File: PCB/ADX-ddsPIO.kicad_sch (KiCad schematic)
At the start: 71 parts, among them J1 Conn_Coaxial, J2 +12V, Q1 BS170, Q2 BS170, Q3 BS170, Q5 BS170, U1 L7805, U2 74LS244, U4 CD2003GB_GP

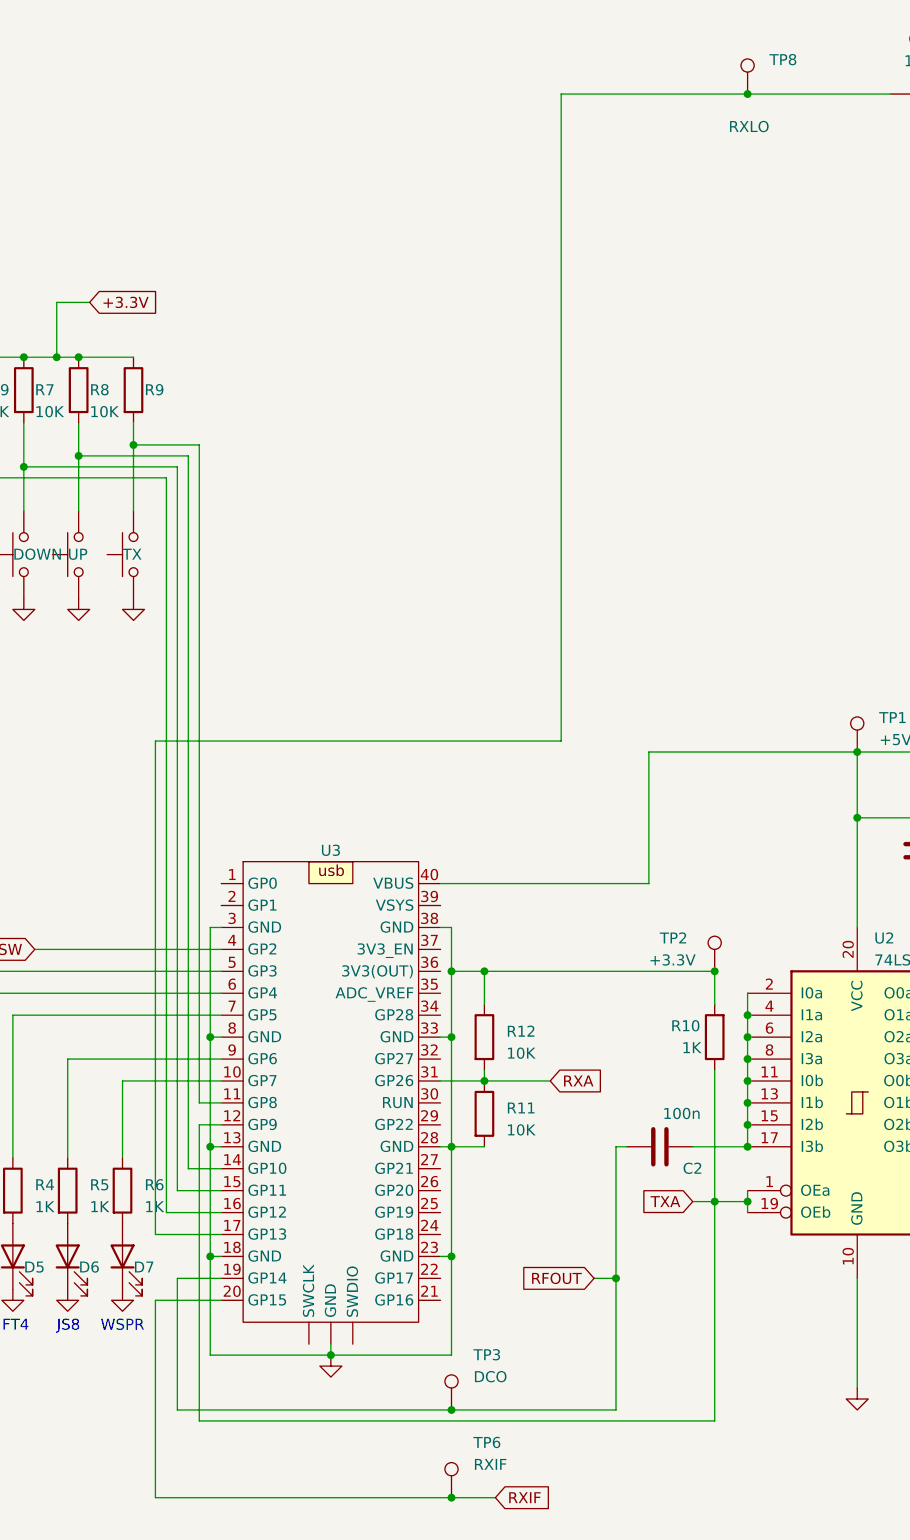
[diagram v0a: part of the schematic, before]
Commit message: dualclk
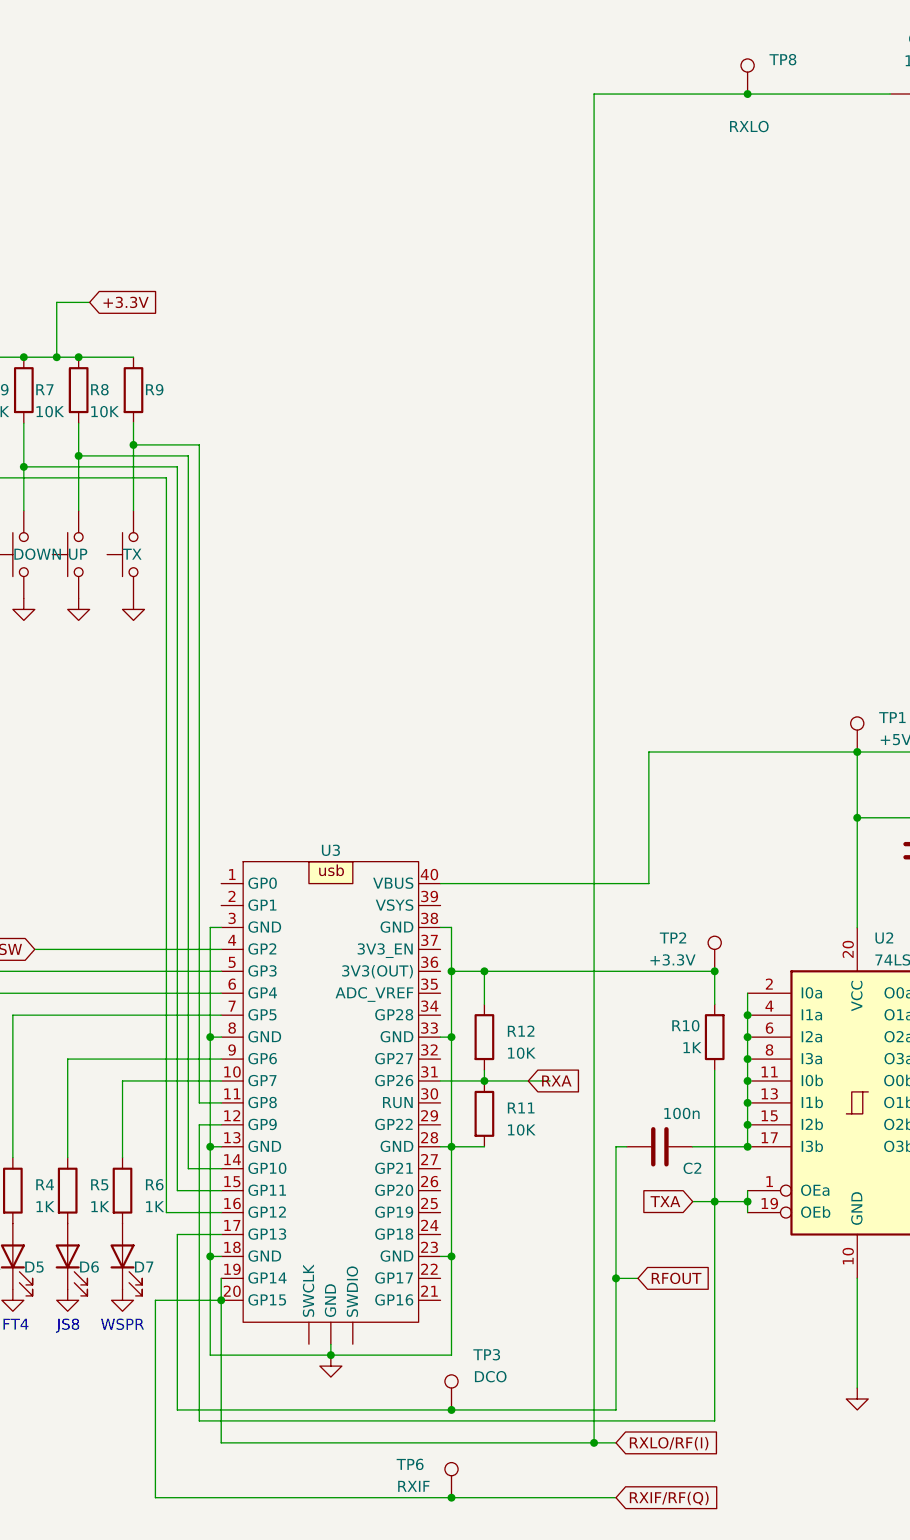
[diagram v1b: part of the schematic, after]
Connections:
- net RXIF is gone; now on net RXIF/RF(Q): TP6.1, U3.20 (GP15)
- net RFOUT: now also U3.17 (GP13); no longer U3.19 (GP14)
- net RXIF/RF(Q): now reaches C20.1, TP8.1
- net RXIF/RF(Q): now also U3.19 (GP14); no longer U3.17 (GP13)
